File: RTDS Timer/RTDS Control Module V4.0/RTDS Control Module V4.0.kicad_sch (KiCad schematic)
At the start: 13 parts, among them J1 PH1-10-UA, K1 G6L-1P_DC5, U1 NE555D, U2 IRLML2060TRPBF

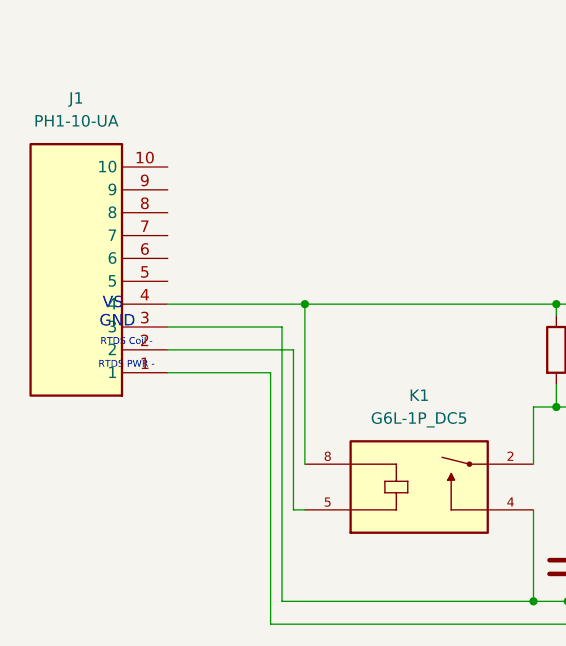
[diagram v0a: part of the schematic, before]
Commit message: Renaming stuff on boards that was wrong
RTDS schematic was totally totally wrong with the pins compared to the PCB
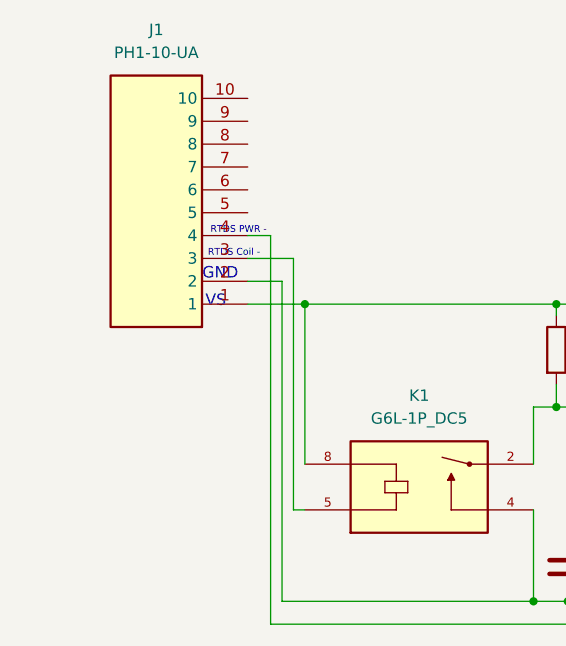
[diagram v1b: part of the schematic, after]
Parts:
- J1: symbol PH1-10-UA:PH1-10-UA -> Symbols:PH1-10-UA
- K1: symbol G6L-1P_DC5:G6L-1P_DC5 -> Symbols:G6L-1P_DC5
- U2: symbol IRLML2060TRPBF:IRLML2060TRPBF -> Symbols:IRLML2060TRPBF
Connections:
- net at K1.8, R1.1, R2.1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: now also J1.1; no longer J1.4
- net at C1.2, C2.2, C3.2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: now also J1.2, J1.4; no longer J1.1, J1.3
- net at K1.5: now also J1.3; no longer J1.2
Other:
- moved on the sheet: J1
